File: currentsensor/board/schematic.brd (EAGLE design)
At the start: 49.5 x 49.4 mm, 41 parts, among them IC1 4050D

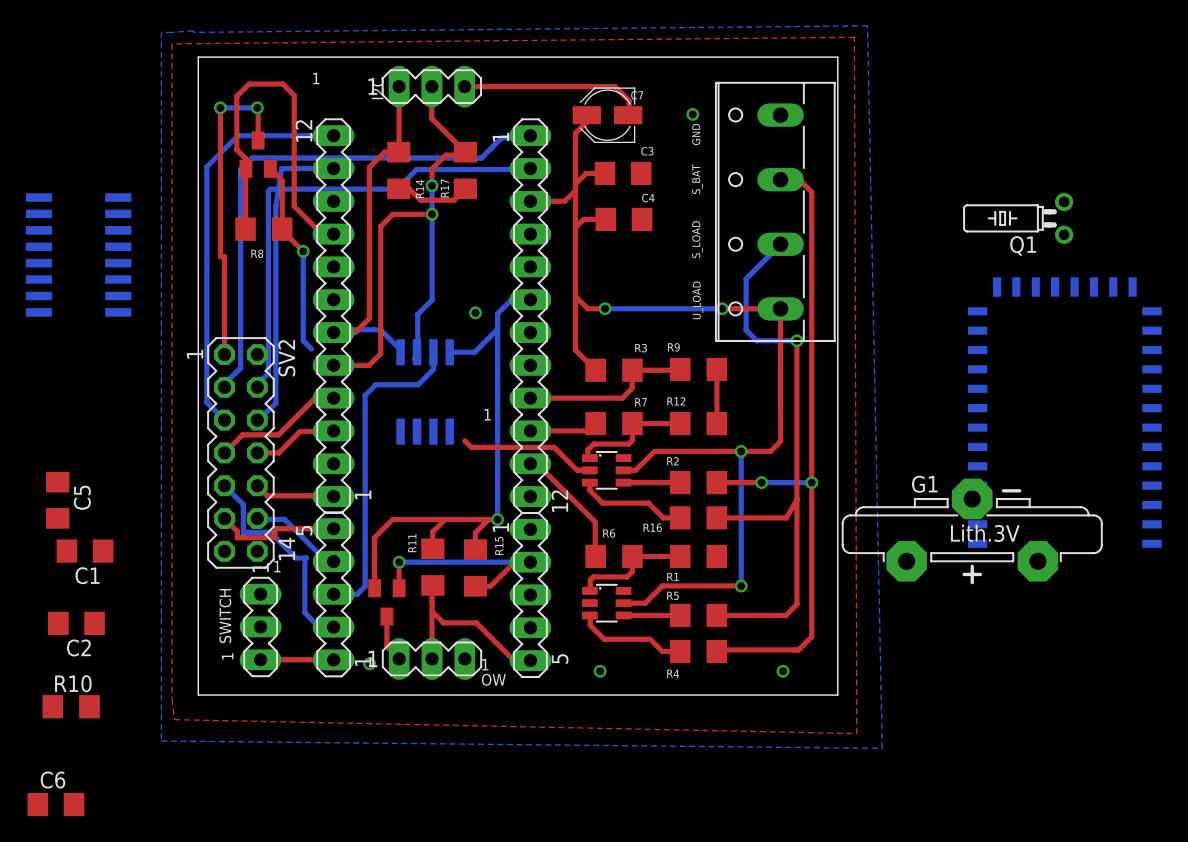
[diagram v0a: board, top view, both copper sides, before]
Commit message: layout
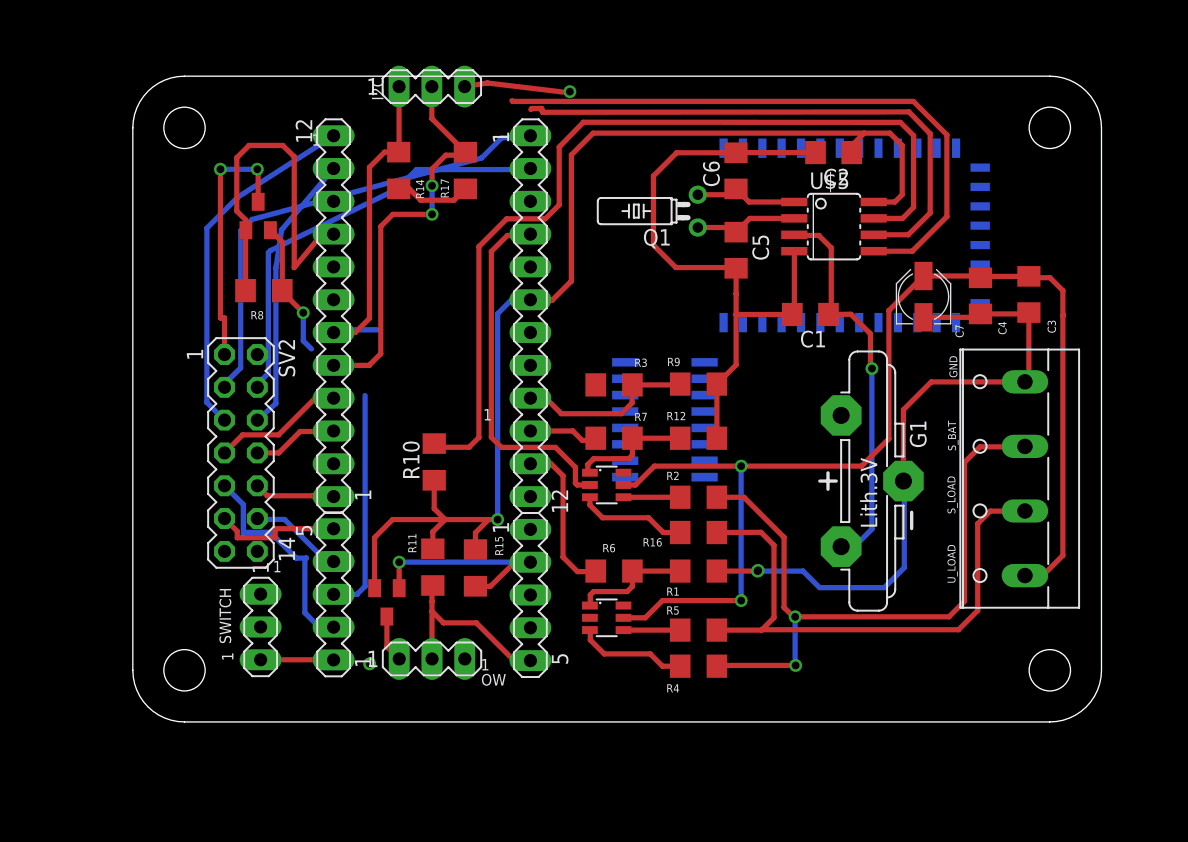
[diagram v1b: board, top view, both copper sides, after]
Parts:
- added PCB1: PCB_DP_RECTANGLE-50X75, dp_pcb:DP5075_V1
- moved C6 72.0 mm to (54.3, 63.6), turned to 90 degrees
- moved C2 69.0 mm to (61.9, 65.0)
- moved C1 59.1 mm to (60.1, 52.5)
- moved C5 56.0 mm to (54.3, 57.4)
- moved IC1 47.1 mm to (48.8, 44.3)
- moved E1 35.7 mm to (53.4, 57.8), turned to 270 degrees
- moved U$5 34.1 mm to (61.9, 59.3), flipped to the top, turned to 270 degrees
- moved R10 33.9 mm to (31.0, 41.0), turned to 90 degrees
- moved C3 32.8 mm to (77.0, 54.0), turned to 90 degrees
- moved Q1 28.4 mm to (51.4, 60.5)
- moved C4 28.2 mm to (73.3, 53.9), turned to 90 degrees
- moved C7 28.2 mm to (68.9, 53.8), turned to 90 degrees
- moved X1 28.0 mm to (75.4, 39.7)
- moved G1 8.45 mm to (65.0, 39.6), turned to 0 degrees
- moved U$3 4.75 mm to (17.3, 60.1)
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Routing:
- net GND: track 29.2 -> 137.2 mm, vias 5 -> 4
- net RTC_IRQ: track 24.9 -> 85.8 mm
- net SDA: track 28.9 -> 74.4 mm
- net +5V: track 62.5 -> 106.6 mm
- net SCL: track 42.8 -> 74.5 mm
- net VBAK: track 0.00 -> 31.0 mm, vias 0 -> 1
- net N$17: track 0.00 -> 8.07 mm
- net N$16: track 0.00 -> 8.06 mm
- net LCD_5V: track 24.8 -> 20.1 mm
- net SPI_CLK: track 40.9 -> 36.8 mm
- net SPI_MISO: track 36.6 -> 32.9 mm
- net SPI_MOSI: track 31.0 -> 27.6 mm
- net SENSE_LOAD: track 46.0 -> 43.4 mm, vias 1 -> 0
- net ADC_I_DISCH: track 9.62 -> 12.2 mm
- net TFT_CS: track 24.2 -> 21.6 mm
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- removed copper zone on layer 1, net GND
- removed copper zone on layer 16, net GND
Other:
- board size 49.5 x 49.4 mm -> 75 x 50 mm
